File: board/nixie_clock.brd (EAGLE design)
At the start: 115 x 55.2 mm, 48 parts, among them U1 AMS1117-5.0, U2 SN74141N

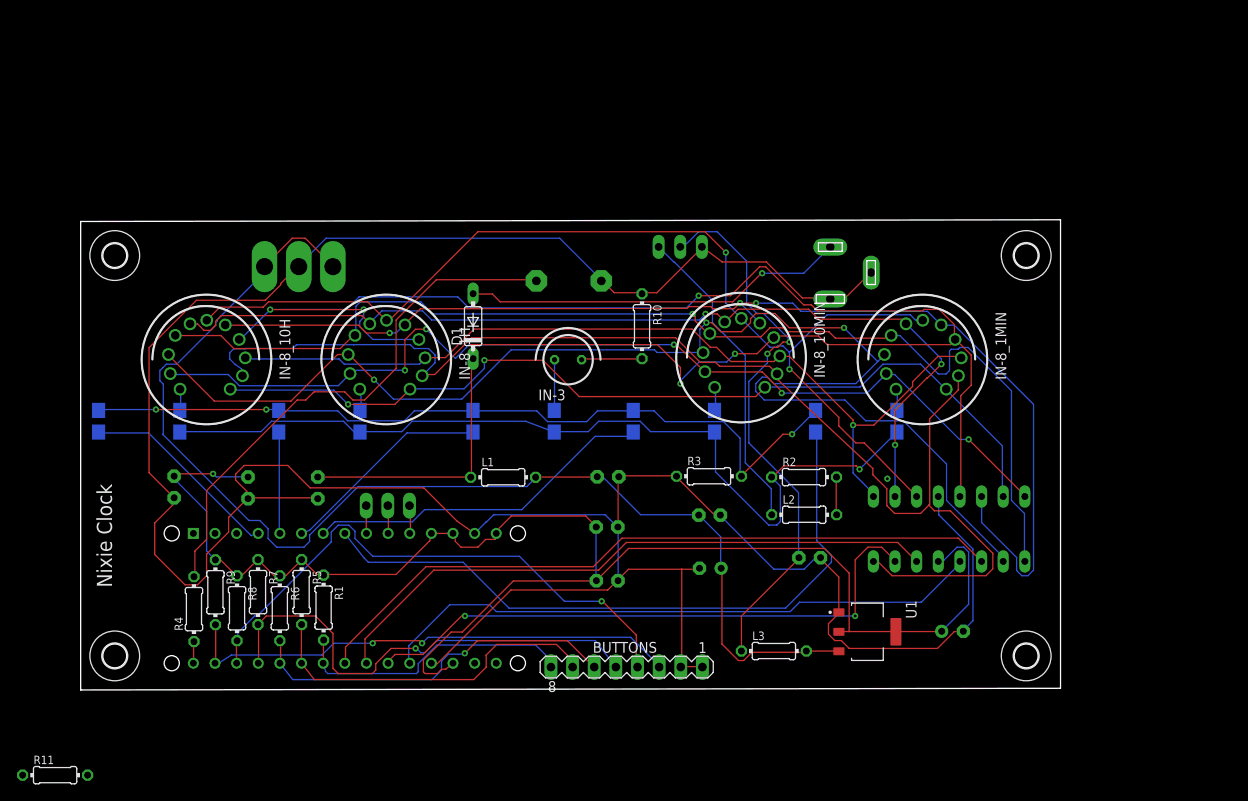
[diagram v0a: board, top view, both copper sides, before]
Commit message: finalized board component layout
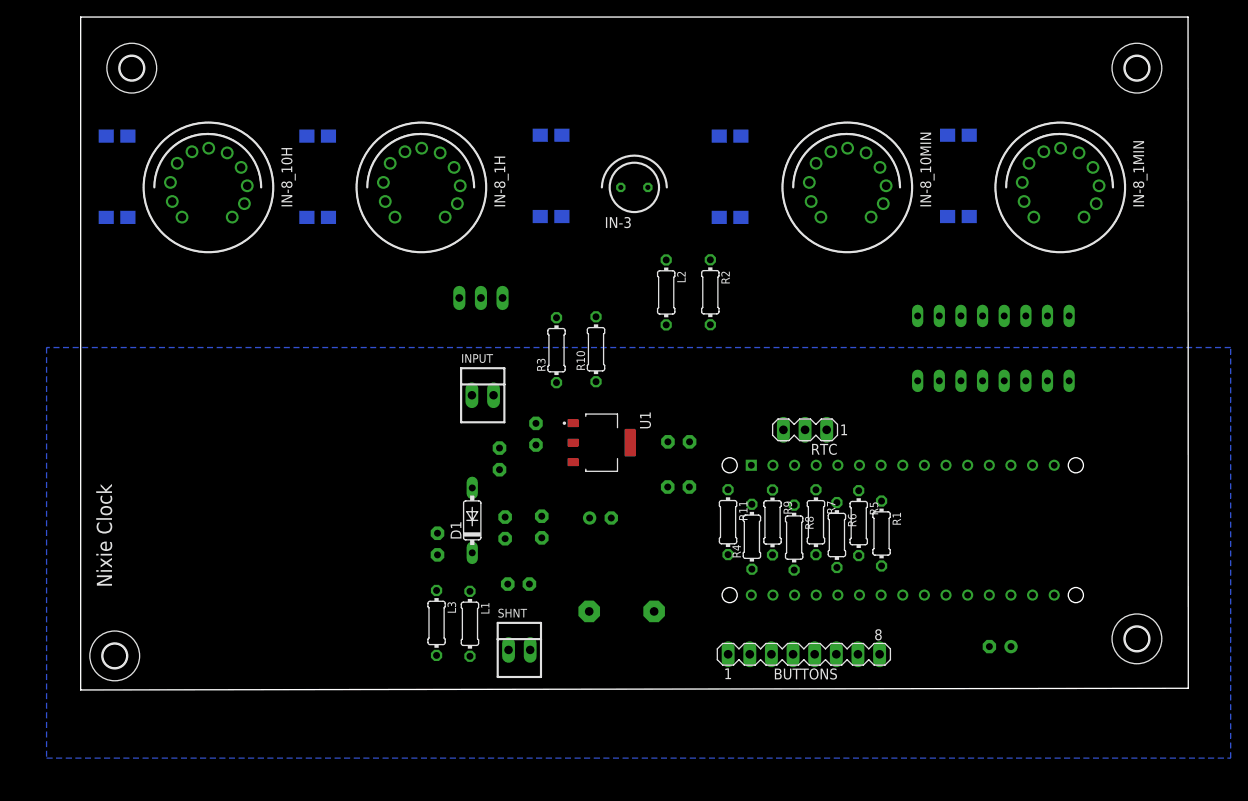
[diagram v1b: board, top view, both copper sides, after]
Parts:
- removed J1: (no value), con-jack:DCJ0303
- added INPUT: 22-23-2021, con-molex:22-23-2021
- SHNT: value (none) -> 22-23-2021; device switch:320-916 -> con-molex:22-23-2021
- moved R11 84.4 mm to (76.0, 19.7), turned to 270 degrees
- moved R1 66.1 mm to (94.0, 18.4)
- moved R4 66.0 mm to (78.8, 18.0)
- moved R7 66.0 mm to (86.3, 19.7)
- moved ARDUINO_NANO1 66.0 mm to (99.0, 18.8)
- moved R6 66.0 mm to (88.8, 18.2)
- moved R8 65.9 mm to (83.8, 17.9)
- moved R9 65.9 mm to (81.2, 19.7)
- moved R5 65.9 mm to (91.3, 19.6)
- moved SHNT 51.9 mm to (51.5, 4.70), flipped to the top, turned to 0 degrees
- moved RTC 49.8 mm to (85.0, 30.5), flipped to the top, turned to 180 degrees
- moved C3 43.7 mm to (41.9, 17.1), turned to 90 degrees
- moved L3 39.7 mm to (41.8, 7.87), turned to 270 degrees
- moved BUZZER 39.3 mm to (63.5, 9.22), turned to 180 degrees
- moved C4 38.3 mm to (49.2, 27.1), turned to 90 degrees
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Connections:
- net +12V: now also SHNT.2; no longer SHNT.1, SHNT.3
- net GND: now also INPUT.2, SHNT.1; no longer J1.1, J1.2, SHNT.2
- net N$1: now also INPUT.1; no longer J1.3
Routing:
- net GND: track 343.6 -> 0.00 mm
- net K4: track 197.0 -> 0.00 mm, vias 5 -> 0
- net +5V: track 177.9 -> 0.00 mm, vias 1 -> 0
- net K9: track 158.5 -> 0.00 mm, vias 3 -> 0
- net K2: track 146.8 -> 0.00 mm
- net +12V: track 142.8 -> 0.00 mm
- net K5: track 137.5 -> 0.00 mm, vias 3 -> 0
- net K8: track 133.7 -> 0.00 mm, vias 1 -> 0
- net K6: track 125.4 -> 0.00 mm, vias 2 -> 0
- net K0: track 117.3 -> 0.00 mm, vias 5 -> 0
- net K7: track 113.4 -> 0.00 mm, vias 3 -> 0
- net K1: track 107.4 -> 0.00 mm, vias 2 -> 0
- net K3: track 104.8 -> 0.00 mm, vias 1 -> 0
- net N$5: track 103.6 -> 0.00 mm, vias 1 -> 0
- net N$16: track 95.4 -> 0.00 mm, vias 3 -> 0
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- added copper zone on layer 16, net GND
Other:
- board size 115 x 55.2 mm -> 130 x 79 mm
